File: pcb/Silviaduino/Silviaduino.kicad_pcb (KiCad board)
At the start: 4 copper layers, 66 x 63.5 mm, 45 parts, among them J1 RTD1 Conn, J10 UEXT_Host, J11 ESP8266, J12 Conn_01x02, J2 RTD 2 Conn, J3 SSR1 Conn, J4 SSR2 Conn, J5 SSR3 Conn, J6 PSSR Conn, J7 PXDCR Conn, J8 Btn Conn, J9 Enc Conn, Q1 2N7002, Q2 2N7002, Q3 2N7002, Q4 BSS138, Q5 BSS138, U1 HT7550-1-SOT89, U2 HT7533-1-SOT89, U3 Teensy4.1, U4 PCF8591, U5 MAX31865xAP, U6 MAX31865xAP

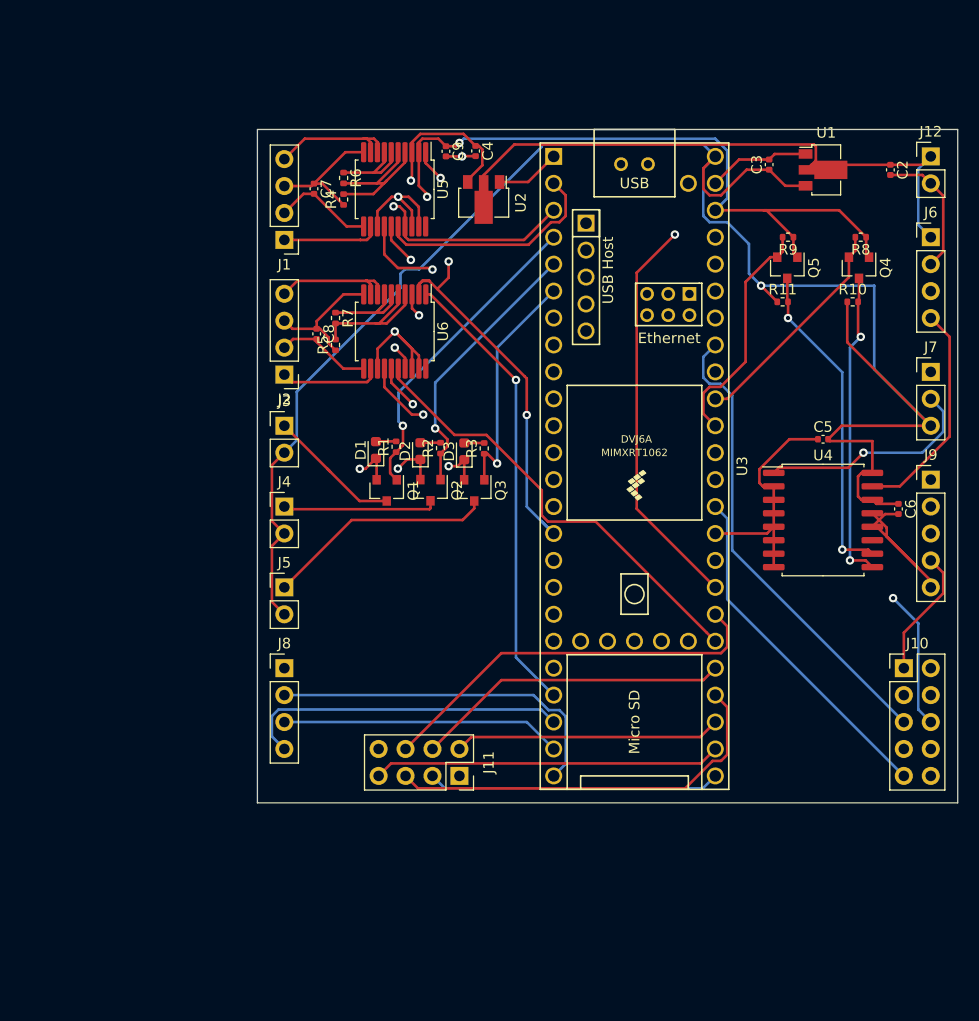
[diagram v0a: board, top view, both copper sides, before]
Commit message: WIP
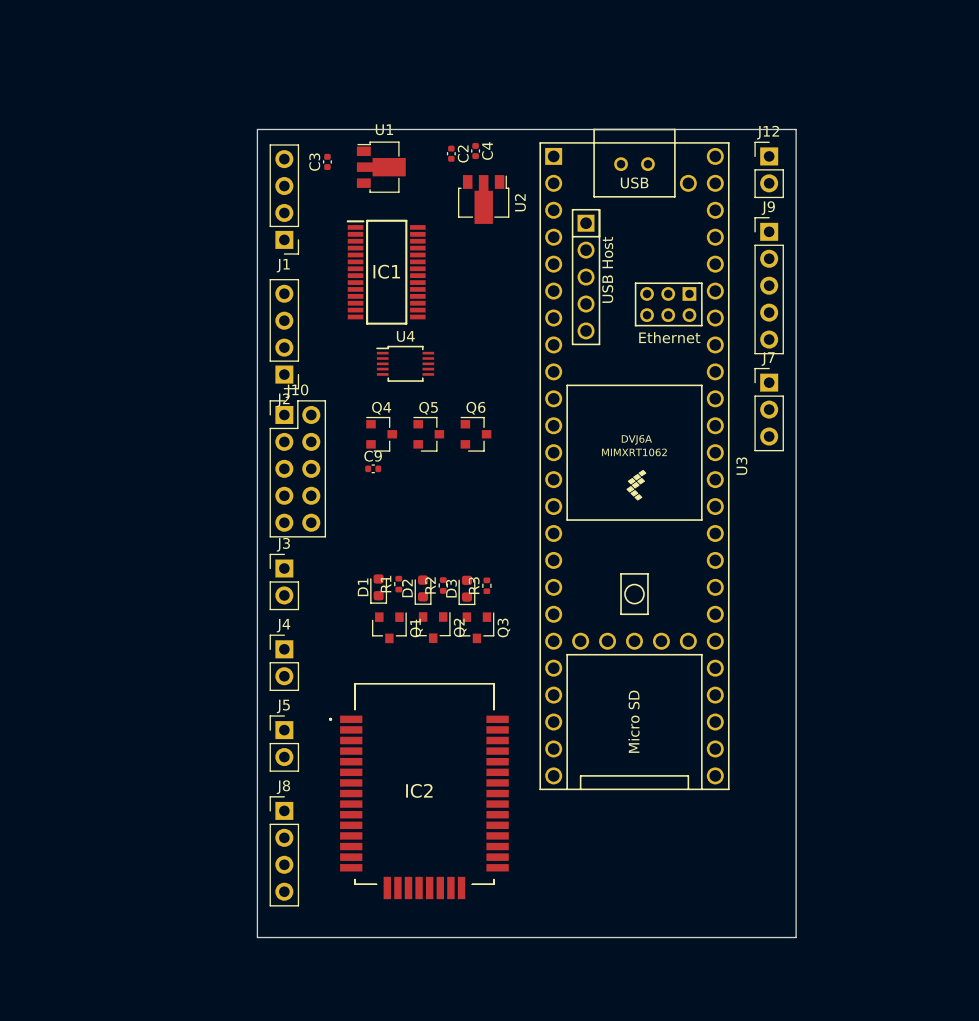
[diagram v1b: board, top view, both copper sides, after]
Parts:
- removed C5, C6: 10 uF, Capacitor_SMD:C_0402_1005Metric
- removed C7, C8: 0.1 uF, Capacitor_SMD:C_0402_1005Metric
- removed J11: ESP8266, Connector_PinSocket_2.54mm:PinSocket_2x04_P2.54mm_Vertical
- removed J6: PSSR Conn, Connector_PinHeader_2.54mm:PinHeader_1x04_P2.54mm_Vertical
- removed R10, R11, R8, R9: 10K, Resistor_SMD:R_0402_1005Metric
- removed R4, R5: 10M, Resistor_SMD:R_0402_1005Metric
- removed R6, R7: 400R, Resistor_SMD:R_0402_1005Metric
- removed U5, U6: MAX31865xAP, Package_SO:SSOP-20_5.3x7.2mm_P0.65mm
- added IC1: ADS1248IPWR, ads1248:SOP65P640X120-28N, F.Cu at (164.6, 64.3)
- added IC2: TTGO_MICRO_32, ttgo:TTGOMICRO32, F.Cu at (168.1, 112.5)
- added Q6: 2N7002, Package_TO_SOT_SMD:SOT-23, F.Cu at (173.0, 79.5)
- Q4, Q5: value BSS138 -> 2N7002
- U4: value PCF8591 -> ADS1015IDGS; footprint Package_SO:SOIC-16W_7.5x10.3mm_P1.27mm -> Package_SO:TSSOP-10_3x3mm_P0.5mm
- moved J10 63.1 mm to (154.9, 77.7)
- moved Q4 47.7 mm to (164.1, 79.5), turned to 0 degrees
- moved U4 42.0 mm to (166.4, 72.9)
- moved C3 41.7 mm to (159.0, 53.9)
- moved U1 41.7 mm to (164.1, 54.4)
- moved C2 41.4 mm to (170.7, 53.1)
- moved Q5 37.3 mm to (168.6, 79.5), turned to 0 degrees
- moved C9 30.7 mm to (163.3, 82.8), turned to 0 degrees
- moved J9 27.9 mm to (200.7, 60.5)
- moved J7 15.3 mm to (200.7, 74.7)
- moved J12 15.2 mm to (200.7, 53.3)
- moved J3 13.5 mm to (154.9, 92.2)
- moved J4 13.5 mm to (154.9, 99.8)
- moved J8 13.5 mm to (154.9, 115.1)
- moved J5 13.5 mm to (154.9, 107.4)
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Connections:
- J7 pad 2: PRES_AIN -> PXDCR_AIN
- Q4 pad 2: I2C_SDA -> SENSOR_I2C_SCL_3V3
- Q4 pad 3: I2C_SDA_5V -> SENSOR_I2C_SCL_5V
- Q5 pad 2: I2C_SCL -> SENSOR_I2C_SDA_3V3
- Q5 pad 3: I2C_SCL_5V -> SENSOR_I2C_SDA_5V
- U3 pad 10: UEXT_TXD -> Net-(U3-Pad10)
- U3 pad 11: Net-(U3-Pad11) -> ESP_RES
- U3 pad 12: UEXT_SSEL -> SENSOR_ADS1248_CS
- U3 pad 13: UEXT_MOSI -> SENSOR_MOSI
- U3 pad 14: UEXT_MISO -> SENSOR_MISO
- U3 pad 16: Net-(U3-Pad16) -> SENSOR_I2C_SCL_3V3
- U3 pad 17: Net-(U3-Pad17) -> SENSOR_I2C_SDA_3V3
- U3 pad 18: TEMP_SPI_MOSI -> ESP_MOSI
- U3 pad 19: TEMP_SPI_SCK -> ESP_SCK
- U3 pad 2: TEMP_SPI_CS0 -> ESP_CS
- U3 pad 20: TEMP_DRDY0 -> ESP_TX
- U3 pad 21: TEMP_DRDY1 -> ESP_RX
- U3 pad 25: ESP8266_RST -> TEENSY_GPIO4
- U3 pad 26: RX_FROM_ESP8266 -> TEENSY_GPIO3
- U3 pad 27: TX_TO_ESP8266 -> TEENSY_GPIO2
- U3 pad 28: ESP8266_CHPD -> SENSOR_EXT2_CS
- U3 pad 29: ESP8266_GPIO0 -> SENSOR_EXT1_CS
- U3 pad 3: TEMP_SPI_MISO -> ESP_MISO
- U3 pad 30: TEMP_SPI_CS1 -> Net-(U3-Pad30)
- U3 pad 31: ESP8266_GPIO2 -> Net-(U3-Pad31)
- U3 pad 32: PROP_SSR_EN -> ESP_GPIO0
- U3 pad 33: Net-(U3-Pad33) -> ESP_BUSY
- U3 pad 35: UEXT_SCK -> SENSOR_SCK
- U3 pad 36: Net-(U3-Pad36) -> SENSOR_ADS1248_START
- U3 pad 37: Net-(U3-Pad37) -> SENSOR_ADS1248_DRDY
- U3 pad 38: I2C_SCL -> TEENSY_GPIO1
- U3 pad 39: I2C_SDA -> TEENSY_GPIO0
- U3 pad 9: UEXT_RXD -> Net-(U3-Pad9)
- U4 pad 1: PRES_AIN -> Net-(U4-Pad1)
- U4 pad 10: I2C_SCL_5V -> SENSOR_I2C_SCL_5V
- U4 pad 2: GND -> SENSOR_ADC_RDY_5V
- U4 pad 4: GND -> PXCDR_AIN
- U4 pad 5: GND -> Net-(TP7-Pad1)
- U4 pad 6: GND -> Net-(TP8-Pad1)
- U4 pad 7: GND -> Net-(TP9-Pad1)
- U4 pad 8: GND -> +5V
- U4 pad 9: I2C_SDA_5V -> SENSOR_I2C_SDA_5V
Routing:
- net TEMP_DVDD: track 188.7 -> 0.00 mm, vias 4 -> 0
- net +5V: track 172.9 -> 0.00 mm, vias 1 -> 0
- net GND: track 111.6 -> 0.00 mm, vias 6 -> 0
- net PROP_SSR_EN: track 64.9 -> 0.00 mm, vias 1 -> 0
- net +9V: track 56.8 -> 0.00 mm
- net TEMP_DRDY0: track 55.1 -> 0.00 mm, vias 1 -> 0
- net TEMP_SPI_MOSI: track 52.2 -> 0.00 mm, vias 2 -> 0
- net UEXT_SSEL: track 52.2 -> 0.00 mm
- net TEMP_SPI_SCK: track 49.8 -> 0.00 mm, vias 2 -> 0
- net UEXT_RXD: track 49.5 -> 0.00 mm
- net UEXT_MOSI: track 46.1 -> 0.00 mm
- net UEXT_TXD: track 44.6 -> 0.00 mm
- net UEXT_SCL: track 44.5 -> 0.00 mm
- net TEMP_DRDY1: track 43.0 -> 0.00 mm, vias 1 -> 0
- net TEMP_SPI_CS1: track 42.5 -> 0.00 mm
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- removed copper zone on In1.Cu, net GND
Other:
- board size 66 x 63.5 mm -> 50.8 x 76.2 mm

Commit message: PCB work
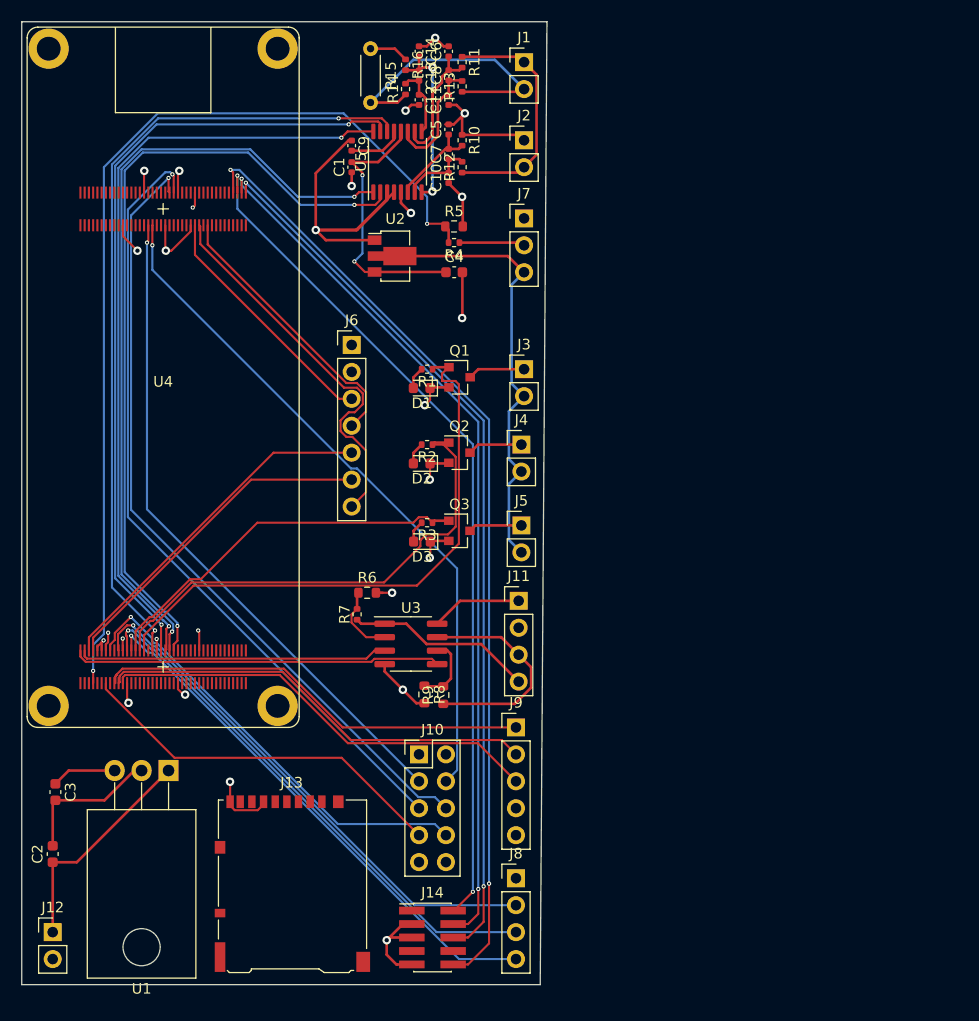
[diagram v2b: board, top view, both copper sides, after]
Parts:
- removed IC1: ADS1248IPWR, ads1248:SOP65P640X120-28N
- removed IC2: TTGO_MICRO_32, ttgo:TTGOMICRO32
- removed Q4, Q5, Q6: 2N7002, Package_TO_SOT_SMD:SOT-23
- added C1: 100 nF, Capacitor_SMD:C_0402_1005Metric, F.Cu at (161.3, 54.4)
- added C10: 10 nF, Capacitor_SMD:C_0402_1005Metric, F.Cu at (170.4, 55.4)
- added C11: 10 nF, Capacitor_SMD:C_0402_1005Metric, F.Cu at (170.4, 48.0)
- added C12: 10 nF, Capacitor_SMD:C_0402_1005Metric, F.Cu at (167.6, 48.0)
- added C13: 100 nF, Capacitor_SMD:C_0402_1005Metric, F.Cu at (167.6, 45.7)
- added C14: 10 nF, Capacitor_SMD:C_0402_1005Metric, F.Cu at (167.6, 43.4)
- added C5: 10 nF, Capacitor_SMD:C_0402_1005Metric, F.Cu at (170.4, 50.8)
- added C6: 10 nF, Capacitor_SMD:C_0402_1005Metric, F.Cu at (170.4, 43.4)
- added C7: 100 nF, Capacitor_SMD:C_0402_1005Metric, F.Cu at (170.4, 53.1)
- added C8: 100 nF, Capacitor_SMD:C_0402_1005Metric, F.Cu at (170.4, 45.7)
- added J11: PSSR Conn, Connector_PinHeader_2.54mm:PinHeader_1x04_P2.54mm_Vertical, F.Cu at (177.0, 95.2)
- added J13: Micro_SD_Card, Connector_Card:microSD_HC_Hirose_DM3AT-SF-PEJM5, F.Cu at (155.7, 121.9)
- added J14: Conn_ARM_JTAG_SWD_10, Connector_PinHeader_1.27mm:PinHeader_2x05_P1.27mm_Vertical_SMD, F.Cu at (168.9, 127.0)
- added J6: Display Conn, Connector_PinHeader_2.54mm:PinHeader_1x07_P2.54mm_Vertical, F.Cu at (161.3, 71.1)
- added R10: 1K, Resistor_SMD:R_0402_1005Metric, F.Cu at (171.7, 51.8)
- added R11: 1K, Resistor_SMD:R_0402_1005Metric, F.Cu at (171.7, 44.5)
- added R12: 1K, Resistor_SMD:R_0402_1005Metric, F.Cu at (171.7, 54.4)
- added R13: 1K, Resistor_SMD:R_0402_1005Metric, F.Cu at (171.7, 46.7)
- added R14: 1K, Resistor_SMD:R_0402_1005Metric, F.Cu at (166.4, 47.0)
- added R15: 680R, Resistor_THT:R_Axial_DIN0204_L3.6mm_D1.6mm_P5.08mm_Horizontal, F.Cu at (163.1, 43.2)
- added R16: 1K, Resistor_SMD:R_0402_1005Metric, F.Cu at (166.4, 44.7)
- added R4: 4K7, Resistor_SMD:R_0402_1005Metric, F.Cu at (170.9, 61.5)
- added R5: 9K1, Resistor_SMD:R_0603_1608Metric, F.Cu at (170.9, 59.9)
- added R6: 9K1, Resistor_SMD:R_0603_1608Metric, F.Cu at (162.8, 94.5)
- added R7: 4K7, Resistor_SMD:R_0402_1005Metric, F.Cu at (161.8, 96.5)
- added R8: 3K6, Resistor_SMD:R_0603_1608Metric, F.Cu at (168.1, 104.1)
- added R9: 6K2, Resistor_SMD:R_0603_1608Metric, F.Cu at (169.9, 104.1)
- added U5: ADS1220xPW, Package_SO:TSSOP-16_4.4x5mm_P0.65mm, F.Cu at (165.6, 53.8)
- C2, C3, C4: footprint Capacitor_SMD:C_0402_1005Metric -> Capacitor_SMD:C_0603_1608Metric
- C9: value 0.1 uF -> 100 nF
- J1, J2: footprint Connector_PinHeader_2.54mm:PinHeader_1x04_P2.54mm_Vertical -> Connector_PinHeader_2.54mm:PinHeader_1x02_P2.54mm_Vertical
- U1: value HT7550-1-SOT89 -> 78S04; footprint Package_TO_SOT_SMD:SOT-89-3 -> Package_TO_SOT_THT:TO-220-3_Horizontal_TabDown
- U3: value Teensy4.1 -> MCP6002-xSN; footprint teensy:Teensy41 -> Package_SO:SOIC-8_3.9x4.9mm_P1.27mm
- U4: value ADS1015IDGS -> Portenta_H7; footprint Package_SO:TSSOP-10_3x3mm_P0.5mm -> Arduino:Arduino_Portenta_H7
- moved J12 99.6 mm to (133.1, 126.5)
- moved C2 76.0 mm to (133.1, 119.1), turned to 90 degrees
- moved C3 64.7 mm to (133.3, 113.3), turned to 270 degrees
- moved U1 60.3 mm to (144.0, 111.3), turned to 180 degrees
- moved J9 52.5 mm to (176.8, 107.2)
- moved J10 34.4 mm to (167.6, 109.7)
- moved J2 31.6 mm to (177.5, 51.8), turned to 0 degrees
- moved C9 30.5 mm to (161.3, 52.3), turned to 270 degrees
- moved J4 29.5 mm to (177.3, 80.5)
- moved J5 29.5 mm to (177.3, 88.1)
- moved J3 29.4 mm to (177.5, 73.4)
- moved J1 28.1 mm to (177.5, 44.5), turned to 0 degrees
- moved J7 27.8 mm to (177.5, 59.2)
- moved U3 26.9 mm to (166.9, 99.3), turned to 0 degrees
- moved Q1 24.5 mm to (171.5, 74.2), turned to 0 degrees
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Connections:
- net PXCDR_AIN renamed Net-(U4-Pad4)
- C2 pad 2: GND -> RTD2IN-
- C3 pad 2: GND -> RTD2IN-
- C4 pad 1: TEMP_VDD -> +3.3VA
- C4 pad 2: GND -> RTD2IN-
- C9 pad 1: TEMP_DVDD -> RTD2IN-
- C9 pad 2: GND -> +3V3
- D1 pad 1: GND -> RTD2IN-
- D2 pad 1: GND -> RTD2IN-
- D3 pad 1: GND -> RTD2IN-
- J1 pad 1: RTD1F- -> ADS1220_IDAC1_RTD1
- J1 pad 2: RTD1IN- -> ADS1220_IDAC1_RREF
- J10 pad 1: TEMP_DVDD -> +3V3
- J10 pad 10: UEXT_SSEL -> UEXT_CS
- J10 pad 2: GND -> RTD2IN-
- J10 pad 3: UEXT_TXD -> UART0_TX
- J10 pad 4: UEXT_RXD -> UART0_RX
- J10 pad 5: UEXT_SCL -> I2C0_SCL
- J10 pad 6: UEXT_SDA -> I2C0_SDA
- J10 pad 7: UEXT_MISO -> SPI5_MISO
- J10 pad 8: UEXT_MOSI -> SPI5_MOSI
- J10 pad 9: UEXT_SCK -> SPI5_SCK
- J12 pad 2: GND -> RTD2IN-
- J2 pad 1: RTD2F- -> RTD2IN-
- J2 pad 2: RTD2IN- -> ADS1220_IDAC1_RTD1
- J7 pad 1: GND -> RTD2IN-
- J8 pad 1: GND -> RTD2IN-
- J9 pad 4: TEMP_DVDD -> +3V3
- J9 pad 5: GND -> RTD2IN-
- Q1 pad 2: GND -> RTD2IN-
- Q2 pad 2: GND -> RTD2IN-
- Q3 pad 2: GND -> RTD2IN-
- U1 pad 1: GND -> +9V
- U1 pad 2: +9V -> RTD2IN-
- U2 pad 1: GND -> RTD2IN-
- U2 pad 2: +9V -> +5V
- U2 pad 3: TEMP_VDD -> +3.3VA
- U3 pad 1: GND -> PSSR_DAC_5V
- U3 pad 2: ESP_CS -> Net-(R6-Pad1)
- U3 pad 3: ESP_MISO -> PSSR_DAC_3V3
- U3 pad 4: SSR1_GATE -> RTD2IN-
- U3 pad 5: SSR2_GATE -> PSSR_EN_3V3
- U3 pad 6: SSR3_GATE -> Net-(R8-Pad1)
- U3 pad 7: Net-(U3-Pad7) -> PSSR_EN_9V
- U3 pad 8: Net-(U3-Pad8) -> +9V
- U4 pad 10: SENSOR_I2C_SCL_5V -> Net-(U4-Pad10)
- U4 pad 2: SENSOR_ADC_RDY_5V -> Net-(U4-Pad2)
- U4 pad 3: GND -> Net-(U4-Pad3)
- U4 pad 8: +5V -> Net-(U4-Pad8)
- U4 pad 9: SENSOR_I2C_SDA_5V -> Net-(U4-Pad9)
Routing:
- net RTD2IN-: track 0.00 -> 136.4 mm, vias 0 -> 24
- net Net-(R4-Pad2): track 0.00 -> 90.9 mm, vias 0 -> 2
- net JTAG_RESET: track 0.00 -> 90.0 mm, vias 0 -> 2
- net JTAG_TDO: track 0.00 -> 83.4 mm, vias 0 -> 2
- net JTAG_TCK: track 0.00 -> 82.6 mm, vias 0 -> 2
- net JTAG_TMS: track 0.00 -> 80.9 mm, vias 0 -> 2
- net ADS1220_DRDY: track 0.00 -> 76.3 mm, vias 0 -> 2
- net I2C0_SDA: track 0.00 -> 75.5 mm, vias 0 -> 1
- net ADS1220_CS: track 0.00 -> 75.3 mm, vias 0 -> 2
- net I2C0_SCL: track 0.00 -> 75.3 mm, vias 0 -> 1
- net SPI1_MOSI: track 0.00 -> 75.1 mm, vias 0 -> 2
- net SPI1_SCLK: track 0.00 -> 74.2 mm, vias 0 -> 2
- net SPI1_MISO: track 0.00 -> 73.1 mm, vias 0 -> 2
- net UART0_RX: track 0.00 -> 65.1 mm, vias 0 -> 1
- net UART0_TX: track 0.00 -> 63.1 mm, vias 0 -> 1
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- added copper zone on In1.Cu, net RTD2IN-
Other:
- board size 50.8 x 76.2 mm -> 49.5 x 90.8 mm
- net class 5V added: clearance 0.1, trace_width 0.25, via_dia 0.8, via_drill 0.4
- net class 9V added: clearance 0.1, trace_width 0.25, via_dia 0.8, via_drill 0.4
- net class Default: clearance 0.199 -> 0.1; trace_width 0.25 -> 0.2; via_dia 0.8 -> 0.4; via_drill 0.4 -> 0.2
- rule trace_clearance: 0.199 -> 0.1
- rule via_min_drill: 0.3 -> 0.2
